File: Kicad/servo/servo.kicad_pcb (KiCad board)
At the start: 2 copper layers, 54.5 x 33 mm, 16 parts, among them J1 pwm, J2 servo, J3 servo, J4 servo, J5 servo, P1 XT60

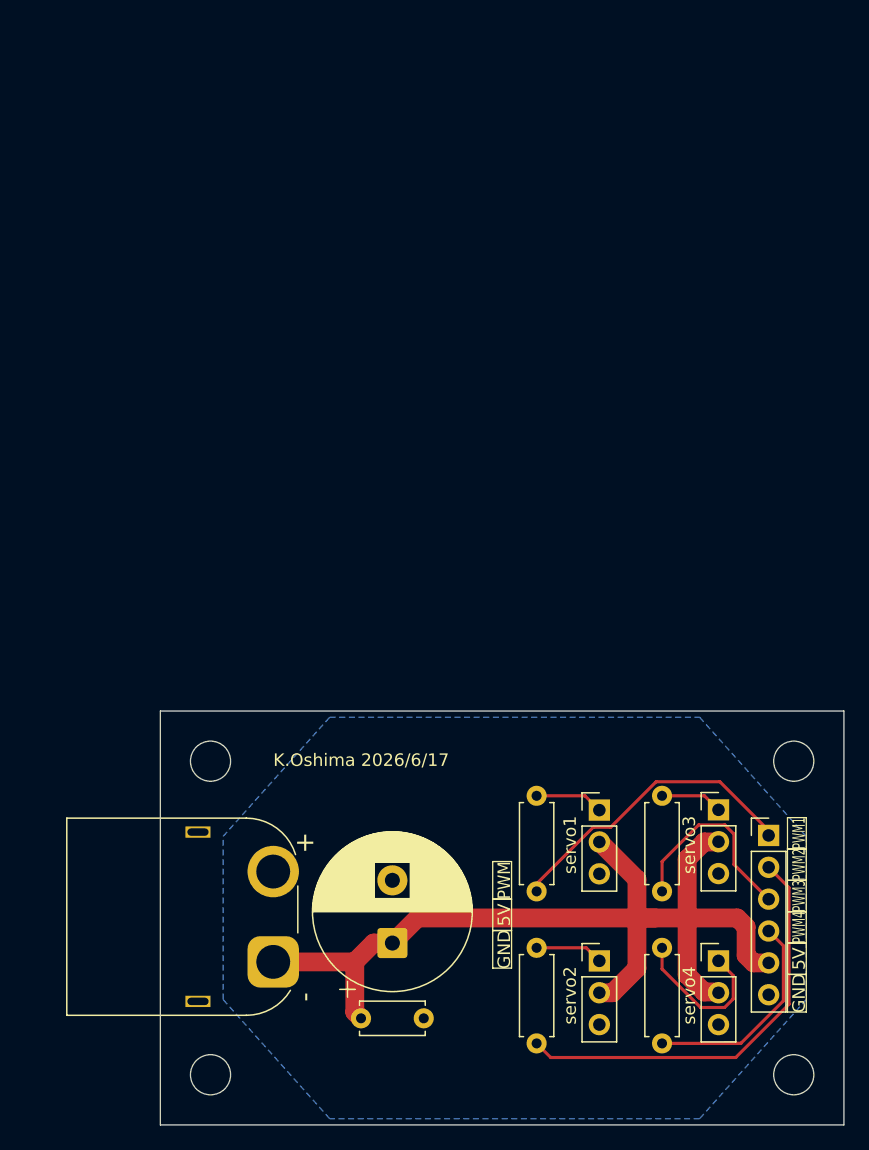
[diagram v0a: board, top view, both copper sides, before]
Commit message: servo回路作成＆PCB用
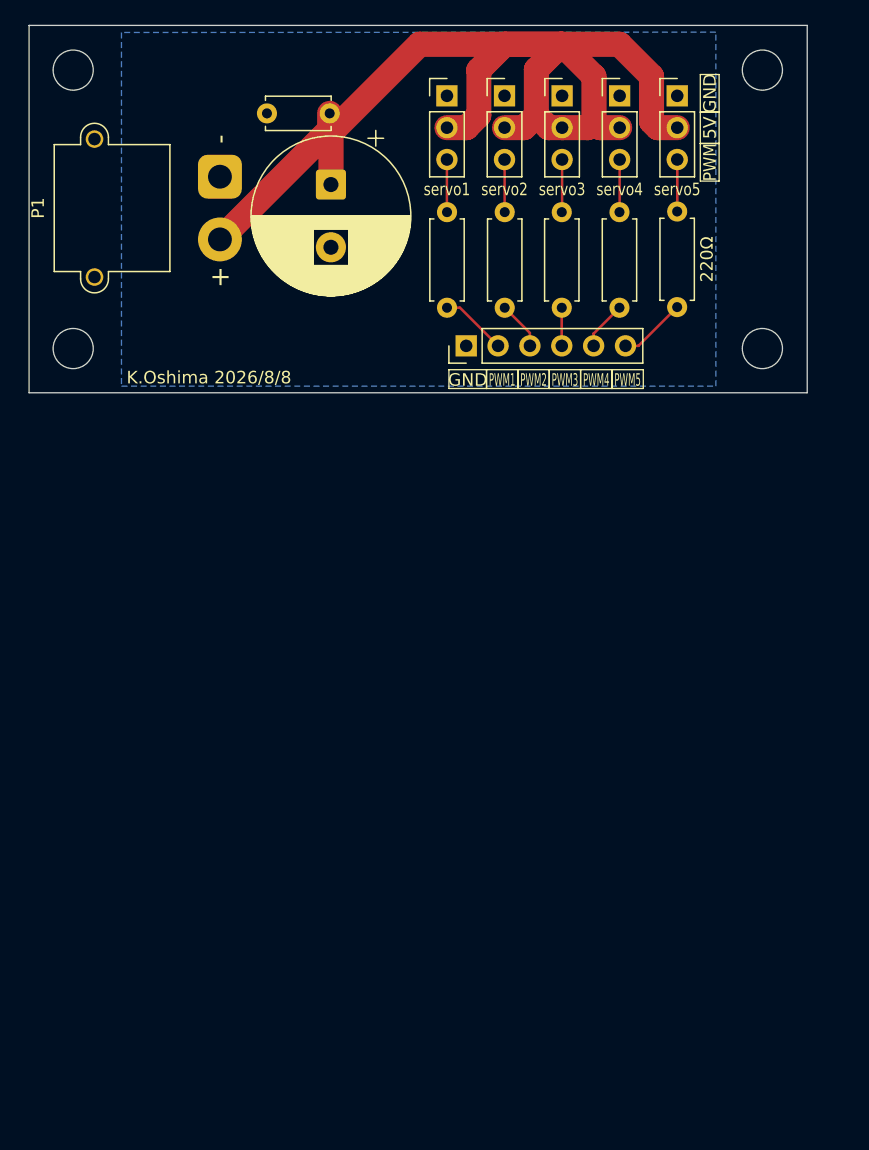
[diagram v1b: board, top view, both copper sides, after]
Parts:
- added J6: servo5, Connector_PinHeader_2.54mm:PinHeader_1x03_P2.54mm_Vertical, F.Cu at (132.7, 64.0)
- added R5: 220Ω, Resistor_THT:R_Axial_DIN0207_L6.3mm_D2.5mm_P7.62mm_Horizontal, F.Cu at (114.4, 80.8)
- J2: value servo -> servo1
- J3: value servo -> servo2
- J4: value servo -> servo3
- J5: value servo -> servo4
- P1: value XT60 -> XT30; footprint Connector_AMASS:AMASS_XT60PW-M_1x02_P7.20mm_Horizontal -> Connector_AMASS:AMASS_XT30PW-M_1x02_P2.50mm_Horizontal
- moved REF** 81.6 mm to (84.5, 84.1)
- moved REF** 80.8 mm to (84.5, 61.9)
- moved C2 72.2 mm to (105.0, 65.3), turned to 180 degrees
- moved REF** 70.5 mm to (139.5, 61.9)
- moved J5 69.4 mm to (128.1, 64.0)
- moved J3 69.4 mm to (118.9, 64.0)
- moved P1 62.7 mm to (96.2, 70.4)
- moved C1 60.7 mm to (105.1, 71.0), turned to -90 degrees
- moved R4 60.0 mm to (119.0, 80.8)
- moved R2 59.0 mm to (128.1, 80.8)
- moved J4 58.3 mm to (123.5, 64.0)
- moved J2 58.2 mm to (114.3, 64.0)
- moved R1 47.9 mm to (132.7, 80.8)
- moved R3 47.2 mm to (123.5, 80.8)
- moved J1 45.9 mm to (115.9, 83.9), turned to 90 degrees
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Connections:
- J1 pad 1: Net-(J1-Pin_1) -> GND
- J1 pad 5: +5V -> Net-(J1-Pin_5)
- J1 pad 6: GND -> Net-(J1-Pin_6)
- J2 pad 1: Net-(J2-Pin_1) -> GND
- J2 pad 3: GND -> Net-(J2-Pin_3)
- J3 pad 1: Net-(J3-Pin_1) -> GND
- J3 pad 3: GND -> Net-(J3-Pin_3)
- J4 pad 1: Net-(J4-Pin_1) -> GND
- J4 pad 3: GND -> Net-(J4-Pin_3)
- J5 pad 1: Net-(J5-Pin_1) -> GND
- J5 pad 3: GND -> Net-(J5-Pin_3)
- P1 pad 1: +5V -> GND
- P1 pad 2: GND -> +5V
- R1 pad 1: Net-(J1-Pin_1) -> Net-(J1-Pin_6)
- R1 pad 2: Net-(J2-Pin_1) -> Net-(J6-Pin_3)
- R2 pad 1: Net-(J1-Pin_2) -> Net-(J1-Pin_5)
- R2 pad 2: Net-(J3-Pin_1) -> Net-(J5-Pin_3)
- R3 pad 1: Net-(J1-Pin_3) -> Net-(J1-Pin_4)
- R3 pad 2: Net-(J4-Pin_1) -> Net-(J4-Pin_3)
- R4 pad 1: Net-(J1-Pin_4) -> Net-(J1-Pin_3)
- R4 pad 2: Net-(J5-Pin_1) -> Net-(J3-Pin_3)
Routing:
- net Net-(J1-Pin_2): track 33.9 -> 5.33 mm
- net Net-(J1-Pin_1): track 24.5 -> 0.00 mm
- net Net-(J1-Pin_4): track 18.4 -> 3.04 mm
- net Net-(J5-Pin_1): track 12.4 -> 0.00 mm
- net Net-(J1-Pin_3): track 16.0 -> 3.87 mm
- net +5V: track 80.6 -> 91.6 mm
- net Net-(J2-Pin_1): track 5.47 -> 0.00 mm
- net Net-(J3-Pin_1): track 5.43 -> 0.00 mm
- net Net-(J1-Pin_6): track 0.00 -> 5.40 mm
- net Net-(J4-Pin_1): track 4.96 -> 0.00 mm
- net Net-(J4-Pin_3): track 0.00 -> 4.21 mm
- net Net-(J5-Pin_3): track 0.00 -> 4.20 mm
- net Net-(J3-Pin_3): track 0.00 -> 4.20 mm
- net Net-(J2-Pin_3): track 0.00 -> 4.20 mm
- net Net-(J6-Pin_3): track 0.00 -> 4.15 mm
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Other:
- board size 54.5 x 33 mm -> 62 x 29.3 mm
- board text added: "K.Oshima 2026/8/8"
- board text added: "Okarobo サーボ用PWM信号分配回路. 6pinからPWMの信号を流す. PWM*はservo*につながる. XTコネクタから電源を供給する."
- board text added: "PWM5"
- board text removed: "K.Oshima 2026/6/17"
- board text removed: "Okarobo サーボ用PWM信号分配回路. 6pinからPWMの信号を流す. PWMxはservoxにつながる. XTコネクタ or 6pinから電源を供給できる."
- board text removed: "servo1"
- board text removed: "servo2"
- board text removed: "servo3"
- board text removed: "servo4"
